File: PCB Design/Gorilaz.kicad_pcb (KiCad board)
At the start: 2 copper layers, 100 x 86 mm, 51 parts, among them CN1 950-D-SMD-DS/02, J1 Conn_01x13, J2 Conn_01x13, J3 Conn_01x13, J4 Conn_01x13, J5 Conn_01x13, J6 Conn_01x13, J7 Battery, J8 Conn_01x05_MountingPin, M1 MountingHole_6.4mm_M6, M3 MountingHole_4.3mm_M4, M4 MountingHole_4.3mm_M4, SW1 RST, U1 SRV05-4, U2 FS8205, U3 DW01A, U4 BQ24075, U5 MAX17048, U8 nRF52840_moko_mk08

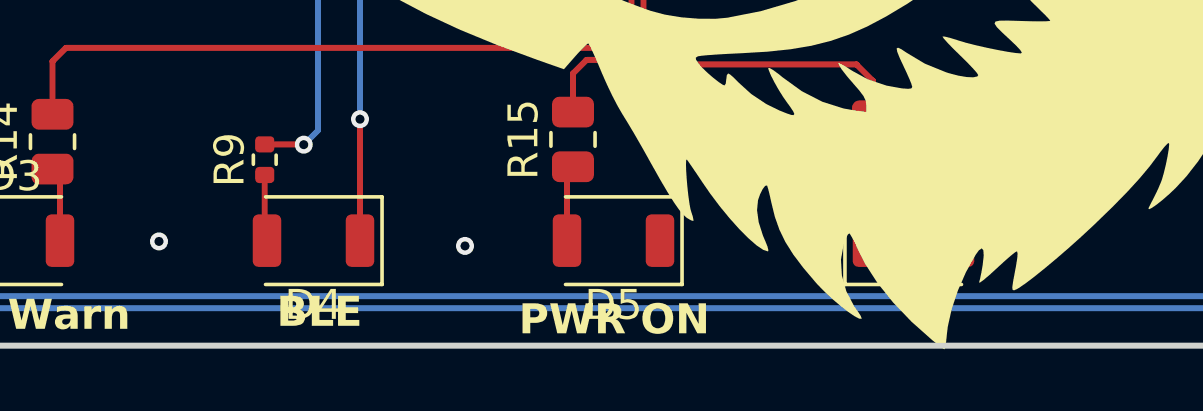
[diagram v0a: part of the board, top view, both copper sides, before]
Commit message: LED update
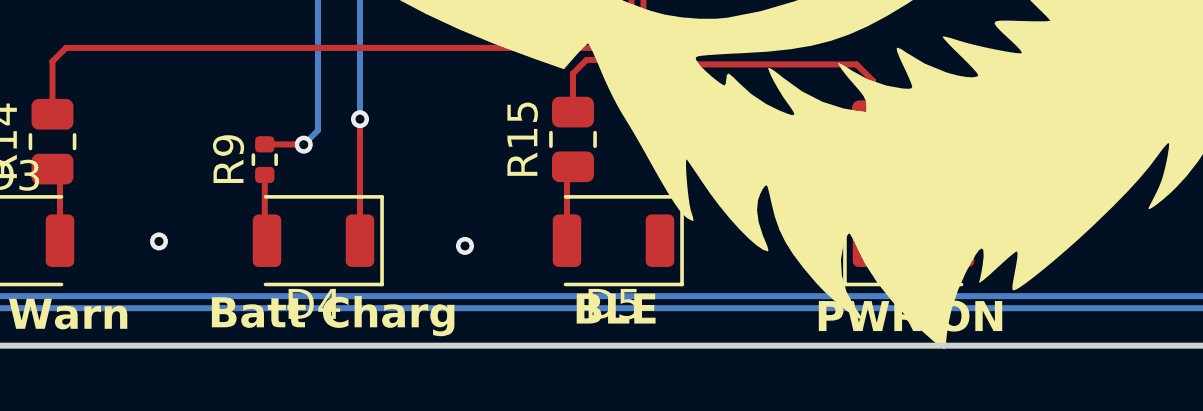
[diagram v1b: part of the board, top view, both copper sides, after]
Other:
- board text added: "Batt Charg"
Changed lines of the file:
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@@
+			)
+		)
+		(model "/home/skullbocks/Documents/Kicad/3D Lib/D_1206_3216Metric.wrl"
+			(offset
+				(xyz 0 0 0)
+			)
+			(scale
+				(xyz 1 1 1)
+			)
+			(rotate
+				(xyz 0 0 0)
 			)
 		)
@@
 	)
 	(gr_text "PWR ON"
-		(at 161.35 124.325 0)
+		(at 171.225 124.25 0)
 		(layer "F.SilkS")
 		(effects
@@
 	)
 	(gr_text "BLE"
-		(at 151.525 124.075 0)
-		(layer "F.SilkS")
-		(effects
+		(at 161.4 124 0)
+		(layer "F.SilkS")
+		(effects
+			(font
+				(size 1 1)
+				(thickness 0.2)
+				(bold yes)
+			)
+		)
+	)
+	(gr_text "Batt Charg"
+		(at 151.975 124.125 0)
+		(layer "F.SilkS")
+		(effects
